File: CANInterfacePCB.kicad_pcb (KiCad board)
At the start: 2 copper layers, 70.9 x 56.9 mm, 16 parts, among them J1 CH1_in, J10 CH1_Debug, J11 CH2_Debug, J2 CH1_out, J3 CH2_in, J4 CH2_out, J5 CH1_EWERT, J6 CH2_EWERT, J7 CH1_PEAK, J8 CH2_PEAK, J9 CH1_CH2_Vector

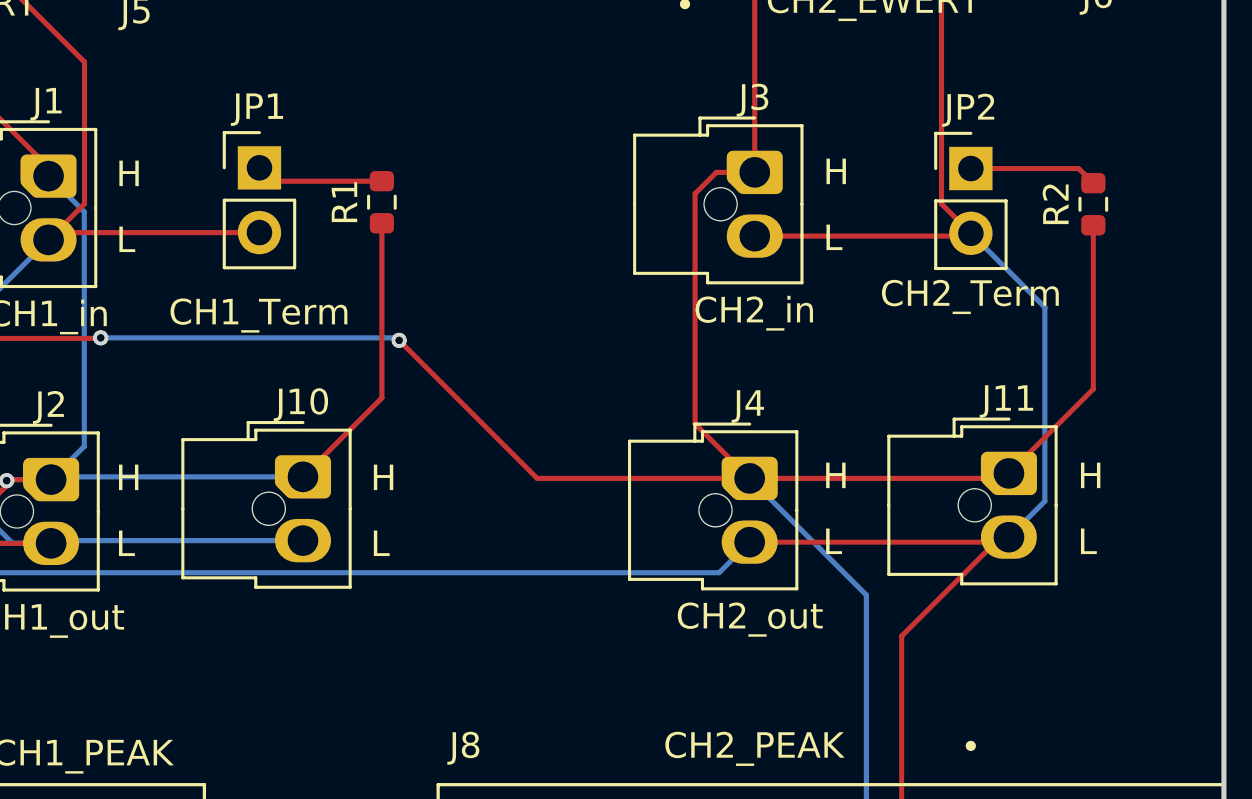
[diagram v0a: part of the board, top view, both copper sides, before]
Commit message: done
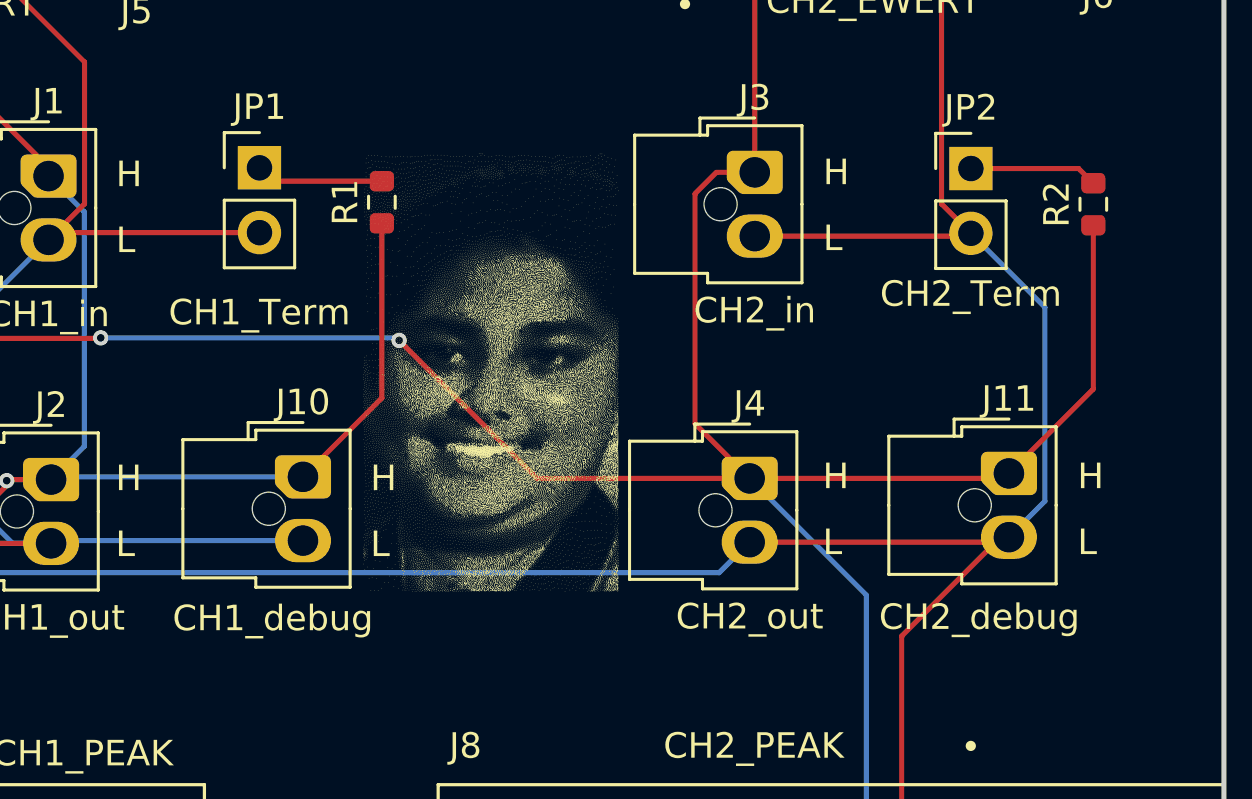
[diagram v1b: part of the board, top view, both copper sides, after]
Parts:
- added G***: LOGO, LOGO, F.Cu at (161.0, 65.7)
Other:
- board text added: "CH1_debug"
- board text added: "CH2_debug"
